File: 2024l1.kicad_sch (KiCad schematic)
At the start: 124 parts, among them IC1 SN74LVC2G04DBVTG4, IC2 SN74LVC2G04DBVTG4, M1 VNH5050A-E, M1C1 680u, M1C2 33n, M1R1 3K3, M1R2 3K3, M1R3 1K, M1R4 1K, M1R5 1K, M1R6 1K, M1R7 1K, M1R8 10K, M1R9 1K5, M1_CONN XT30, M2 VNH5050A-E, M2C2 33n, M2C2 680u, M2R1 3K3, M2R2 3K3, M2R3 1K, M2R4 1K, M2R5 1K, M2R6 1K, M2R7 1K, M2R8 10K, M2R9 1K5, M2_CONN XT30, M3 VNH5050A-E, M3C1 680u, M3C2 33n, M3R1 3K3, M3R2 3K3, M3R3 1K, M3R4 1K, M3R5 1K, M3R6 1K, M3R7 1K, M3R8 10K, M3R9 1K5, M3_CONN XT30, M4 VNH5050A-E, M4C1 680u, M4C2 33n, M4R1 3K3, M4R2 3K3, M4R3 1K, M4R4 1K, M4R5 1K, M4R6 1K, M4R7 1K, M4R8 10K, M4R9 1K5, M4_CONN XT30, U1 3V3 Buck, U2 5V Buck

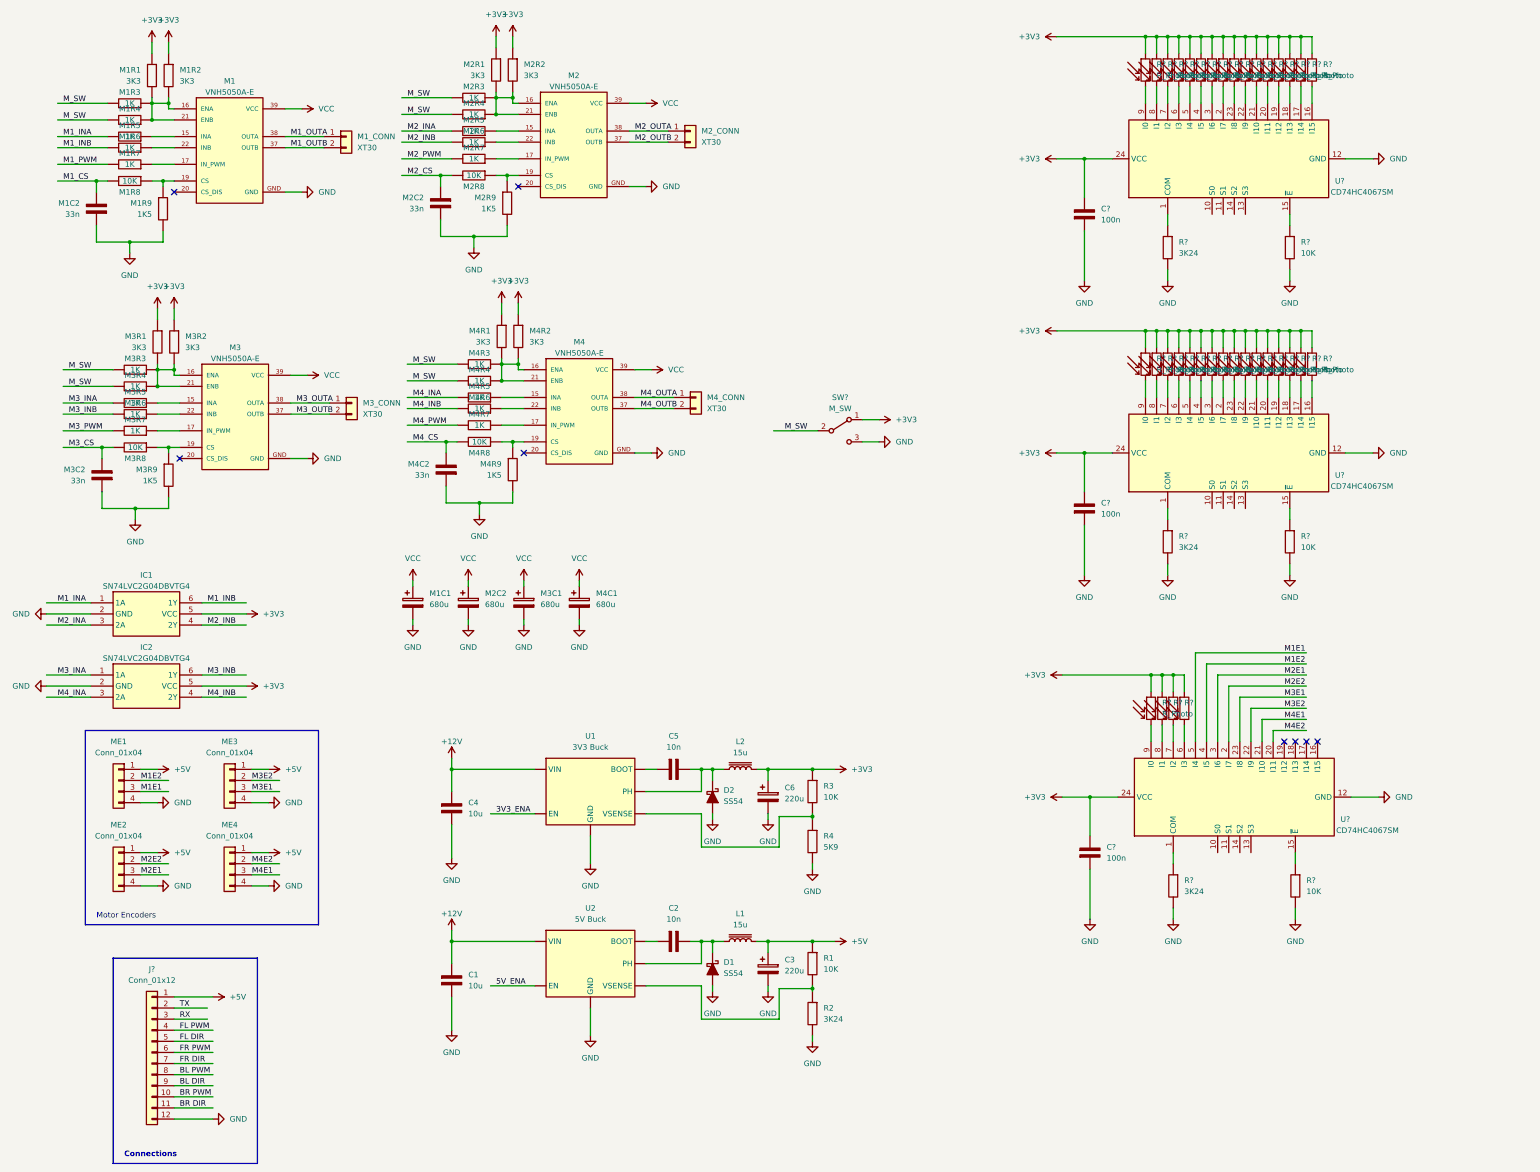
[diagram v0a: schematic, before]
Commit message: split files
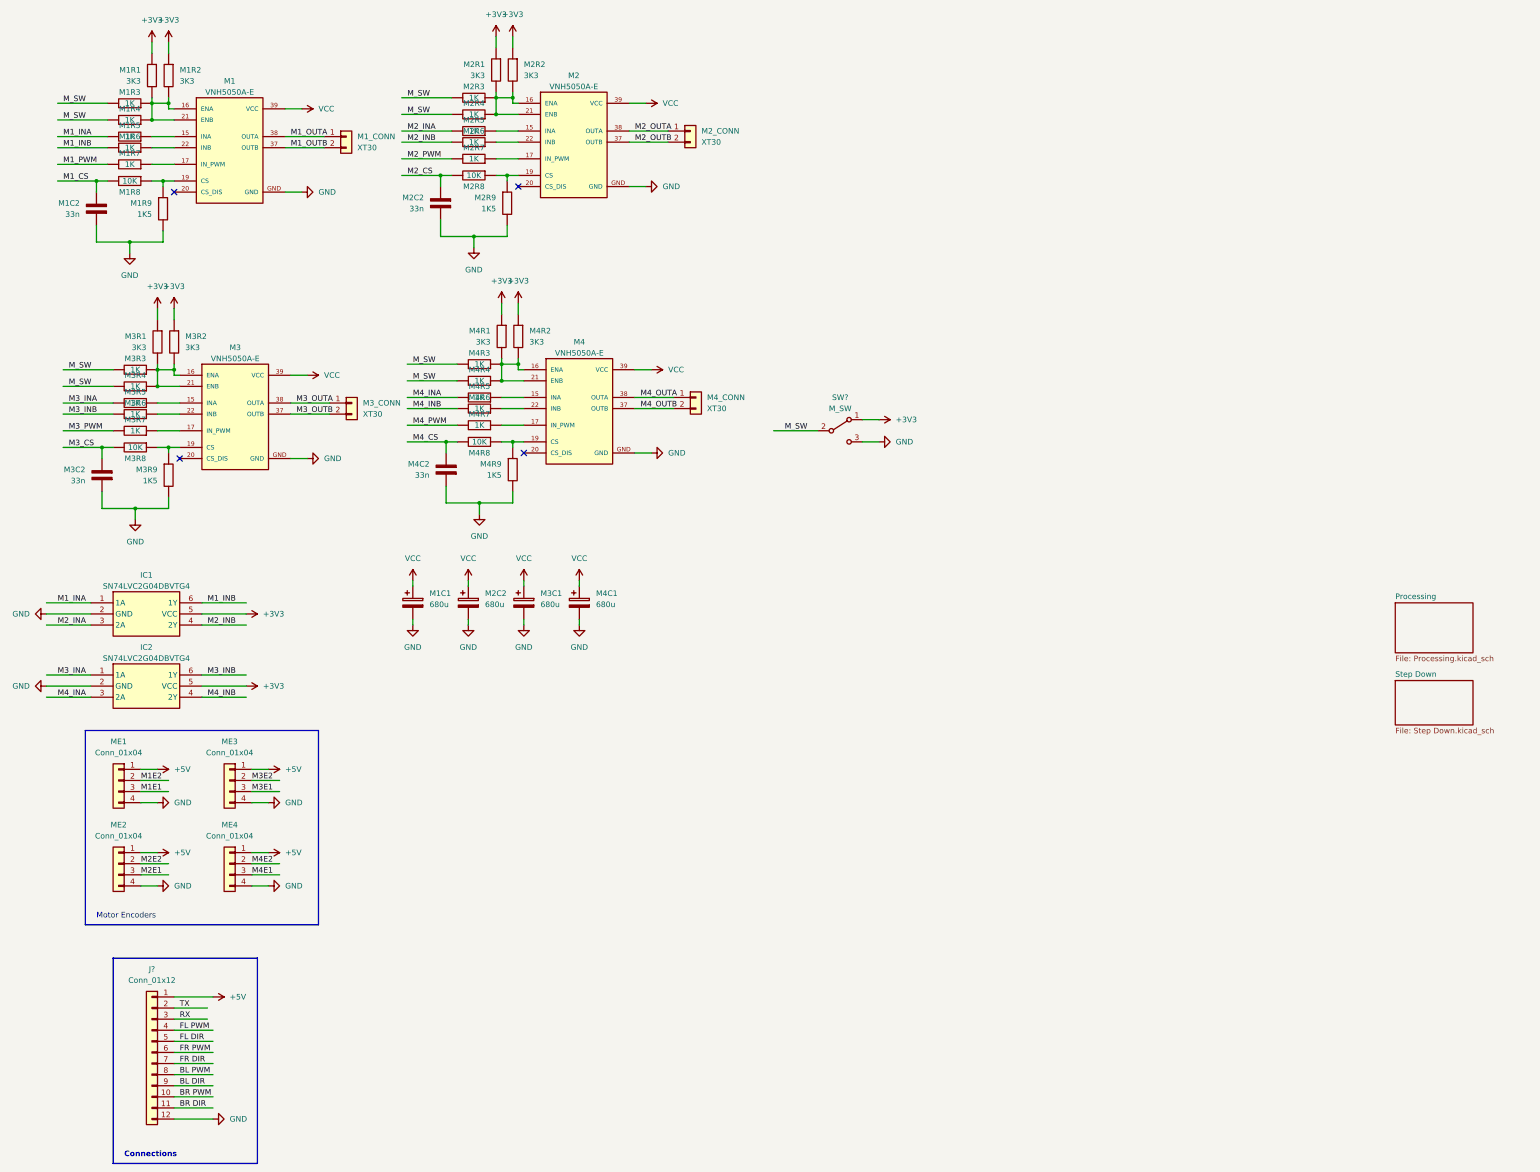
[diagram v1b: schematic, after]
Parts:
- removed C1, C4: 10u, symbol vincent:C
- removed C2, C5: 10n, symbol vincent:C
- removed C3, C6: 220u, symbol vincent:C_Polarized
- removed C? (x3): 100n, symbol vincent:C
- removed D1, D2: SS54, symbol vincent:D_Schotty
- removed L1, L2: 15u, symbol vincent:L_Iron
- removed R1, R3, R? (x3): 10K, symbol vincent:R
- removed R2, R? (x3): 3K24, symbol vincent:R
- removed R4: 5K9, symbol vincent:R
- removed R? (x36): R_Photo, symbol Device:R_Photo
- removed U1: 3V3 Buck, symbol vincent:TPS5430
- removed U2: 5V Buck, symbol vincent:TPS5430
- removed U? (x3): CD74HC4067SM, Package_SO:SSOP-24_5.3x8.2mm_P0.65mm, symbol 74xx:CD74HC4067SM
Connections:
- no-connect marks 8 -> 4
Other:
- added sheet Processing (Processing.kicad_sch)
- added sheet Step Down (Step Down.kicad_sch)

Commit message: stm32
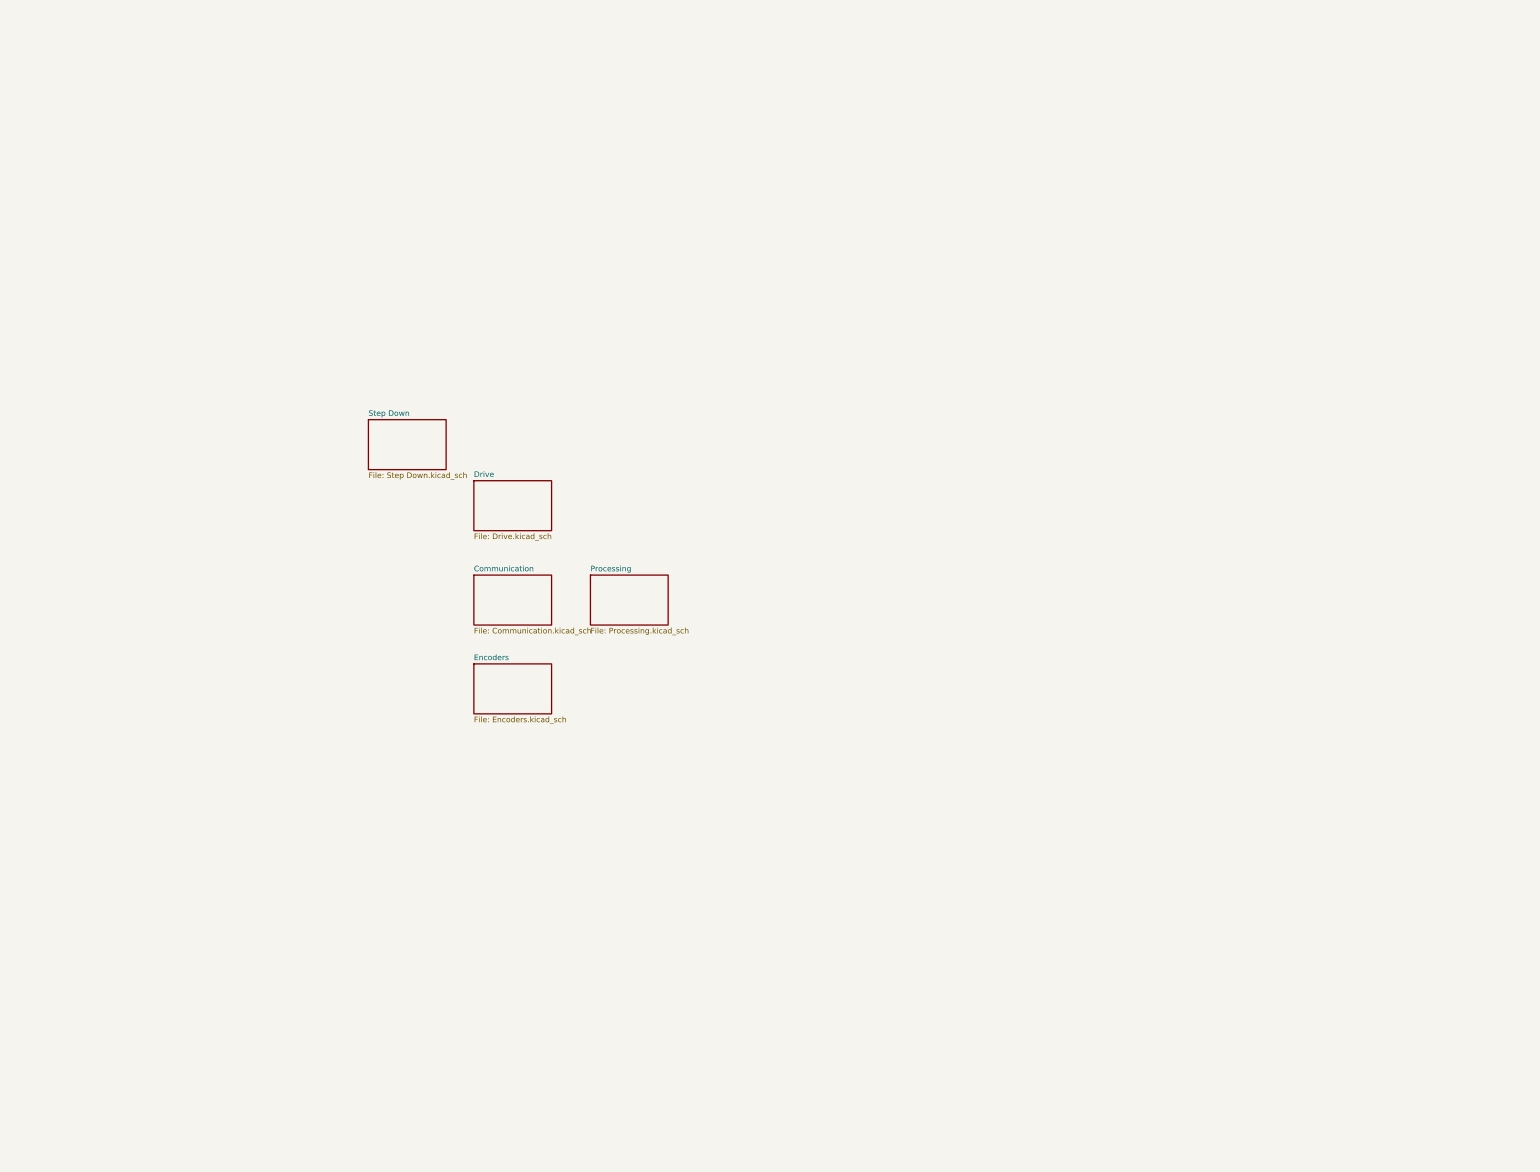
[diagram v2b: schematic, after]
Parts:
- removed IC1, IC2: SN74LVC2G04DBVTG4, SOT95P280X145-6N, symbol vincent:SN74LVC2G04DBVTG4
- removed J?: Conn_01x12, symbol Connector_Generic:Conn_01x12
- removed M1, M2, M3, M4: VNH5050A-E, footprints:SOP50P1030X247-39N, symbol vincent:VNH5050A-E
- removed M1C1, M2C2, M3C1, M4C1: 680u, symbol vincent:C_Polarized
- removed M1C2, M2C2, M3C2, M4C2: 33n, symbol vincent:C
- removed M1R1, M1R2, M2R1, M2R2, M3R1, M3R2, M4R1, M4R2: 3K3, symbol vincent:R
- removed M1R3, M1R4, M1R5, M1R6, M1R7, M2R3, M2R4, M2R5, M2R6, M2R7, M3R3, M3R4, M3R5, M3R6, M3R7, M4R3, M4R4, M4R5, M4R6, M4R7: 1K, symbol vincent:R
- removed M1R8, M2R8, M3R8, M4R8: 10K, symbol vincent:R
- removed M1R9, M2R9, M3R9, M4R9: 1K5, symbol vincent:R
- removed M1_CONN, M2_CONN, M3_CONN, M4_CONN: XT30, symbol Connector_Generic:Conn_01x02
- removed ME1, ME2, ME3, ME4: Conn_01x04, symbol Connector_Generic:Conn_01x04
- removed SW?: M_SW, symbol Switch:SW_SPDT
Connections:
- no-connect marks 4 -> 0
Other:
- added sheet Communication (Communication.kicad_sch)
- added sheet Drive (Drive.kicad_sch)
- added sheet Encoders (Encoders.kicad_sch)
- note removed: "Connections"
- note removed: "Motor Encoders"
